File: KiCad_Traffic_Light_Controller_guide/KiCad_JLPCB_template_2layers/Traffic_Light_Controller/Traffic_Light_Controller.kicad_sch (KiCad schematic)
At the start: 64 parts, among them J1 Conn_02x08_Odd_Even, J2 Conn_02x08_Odd_Even, J3 Conn_02x05_Odd_Even, J4 +5V, SW1 RST, SW2 OVR, SW3 EN, U1 SM420561N, U2 SM420561N, U3 LM1117DT-3.3

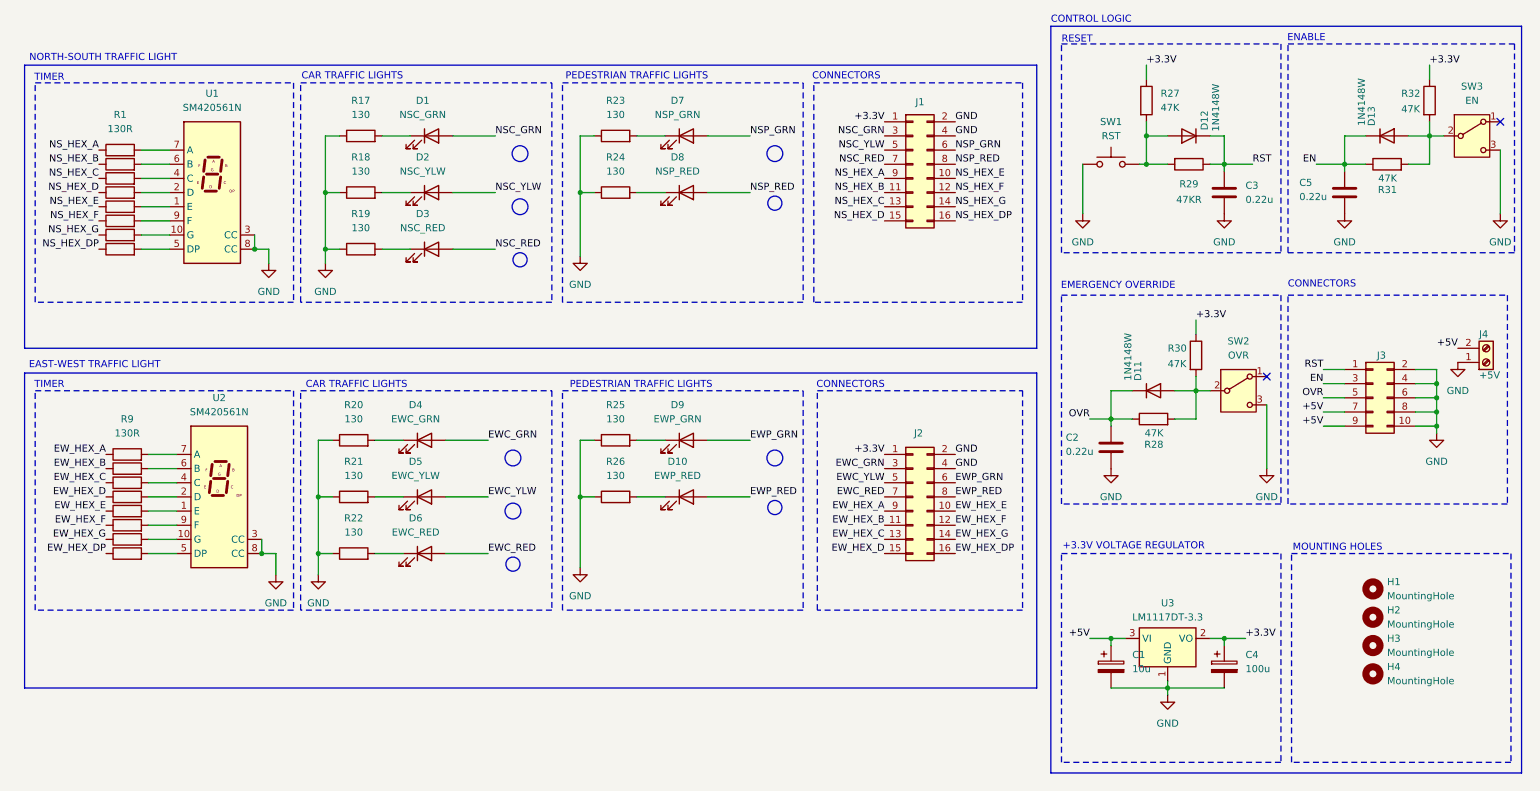
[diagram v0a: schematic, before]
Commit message: commit
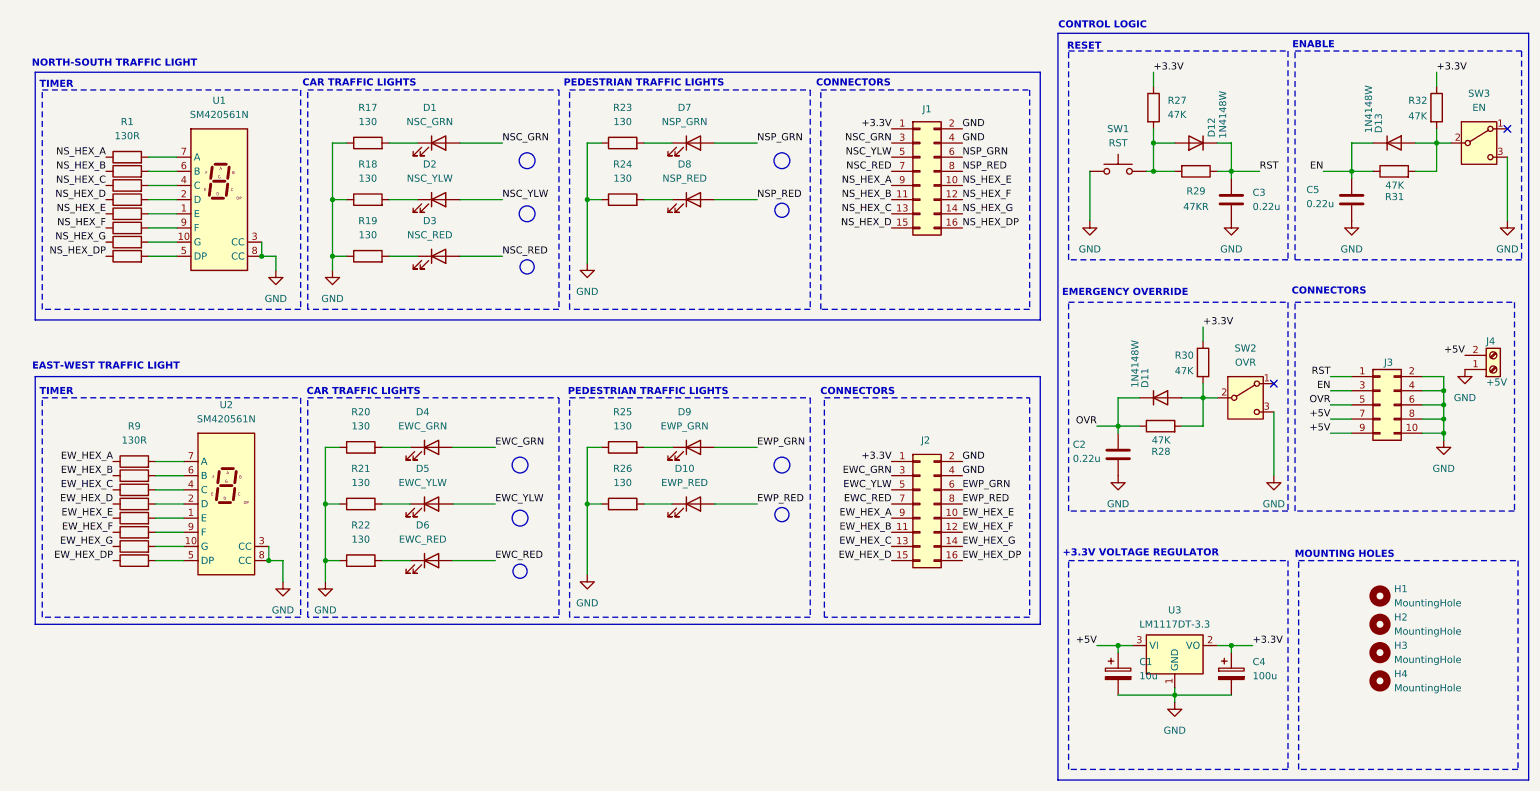
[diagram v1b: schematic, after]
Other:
- moved on the sheet: C1, C2, C3, C4, C5, D1, D10, D11, D12, D13, D2, D3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
